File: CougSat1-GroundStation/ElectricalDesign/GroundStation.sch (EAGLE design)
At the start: 0 parts

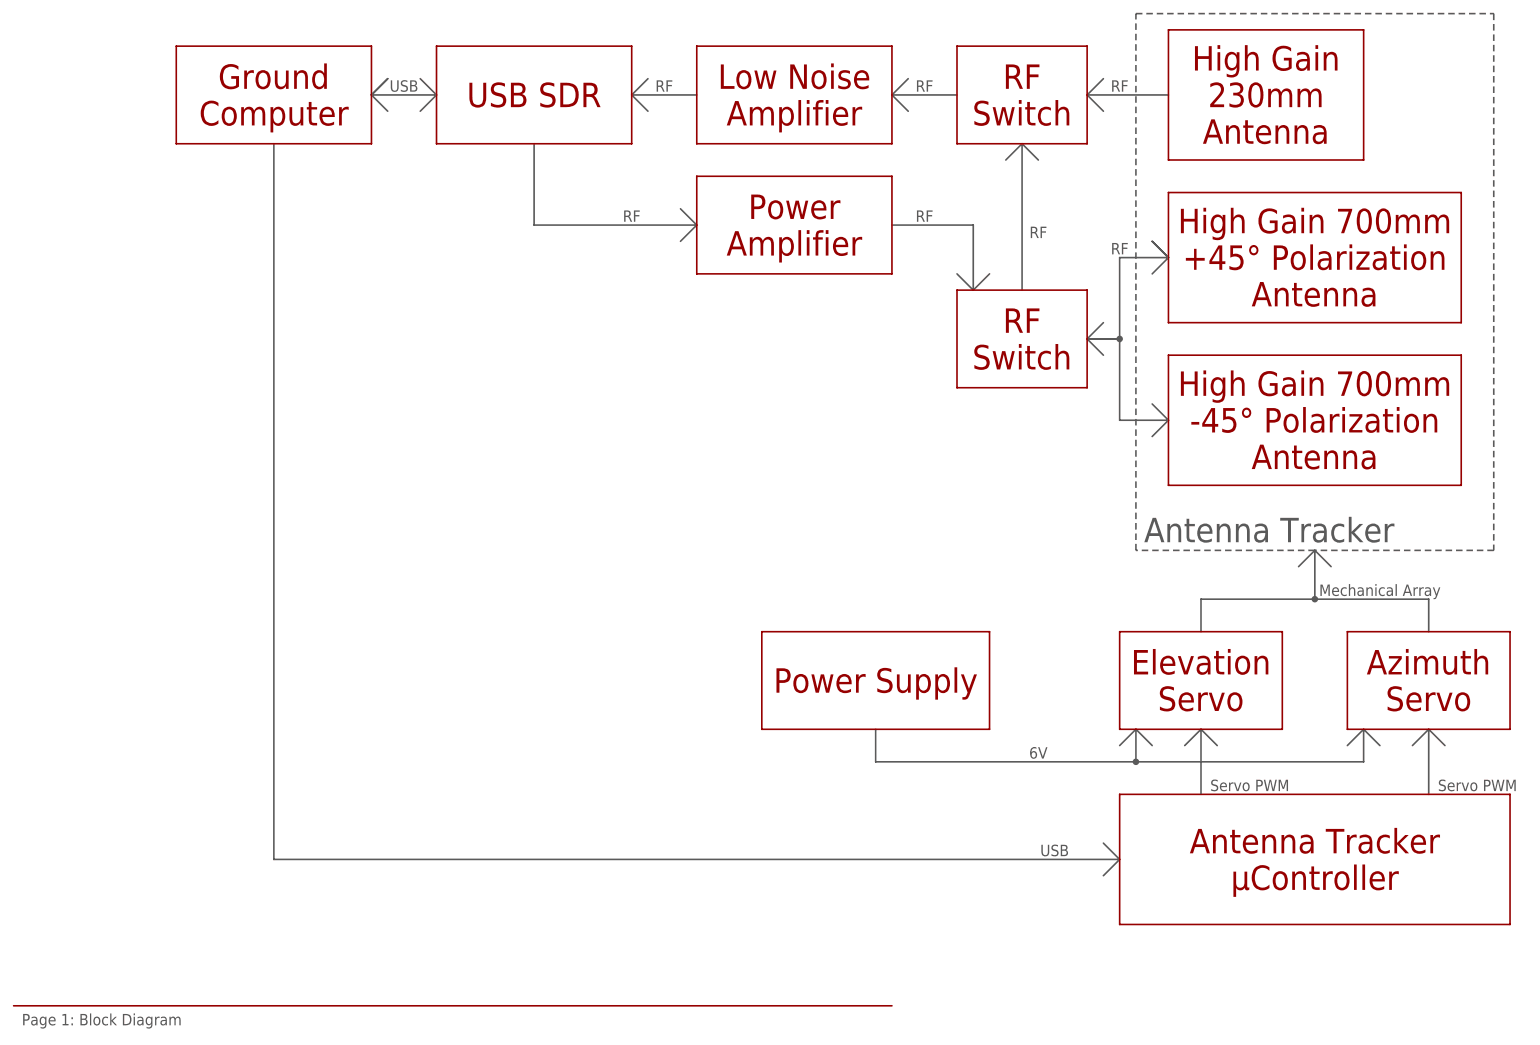
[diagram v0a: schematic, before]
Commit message: Analyzed Link Budget
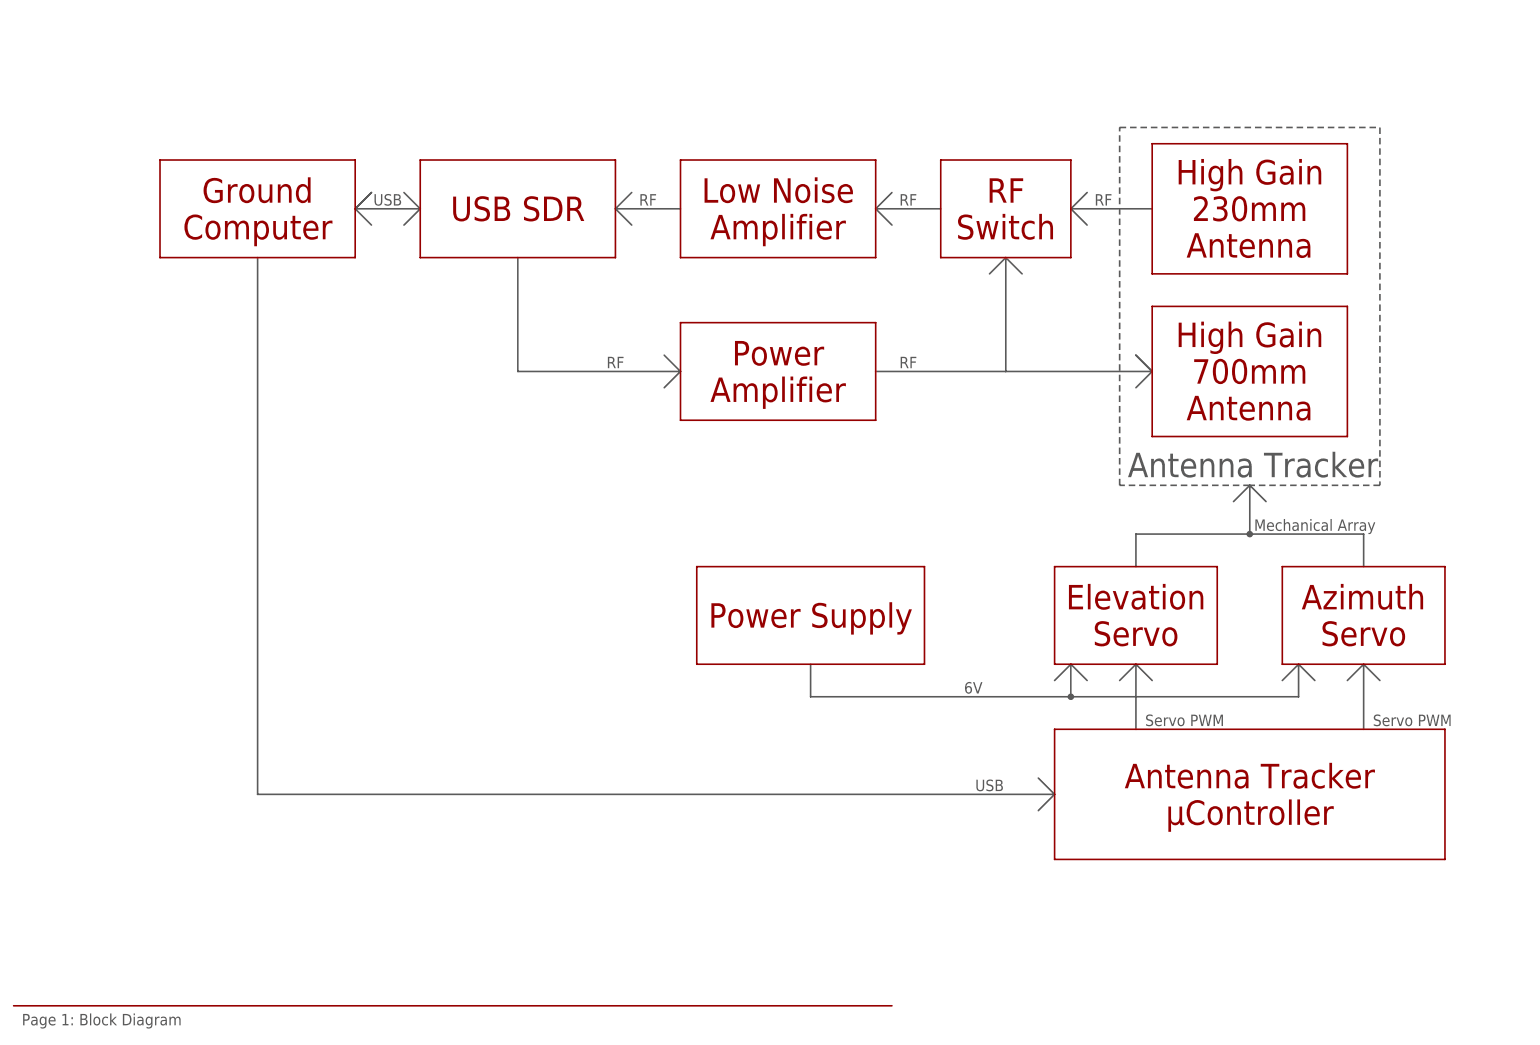
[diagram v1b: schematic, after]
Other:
- note added: "High Gain 700mm Antenna"
- note removed: "High Gain 700mm +45° Polarization Antenna"
- note removed: "High Gain 700mm -45° Polarization Antenna"
